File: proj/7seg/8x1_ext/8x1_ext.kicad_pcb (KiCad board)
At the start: 2 copper layers, 100 x 19 mm, 44 parts, among them J1 Conn_01x03_Pin, J2 grove, J3 UART, J4 UART, J9 USB_C, SW1 SW_Push, U1 74HC595, U10 D168K, U11 MCU_DISP, U12 MCU_CTL, U13 CH340E, U14 CH340K, U2 74HC595, U3 D168K, U4 D168K, U5 D168K, U6 D168K, U7 D168K, U8 D168K, U9 D168K

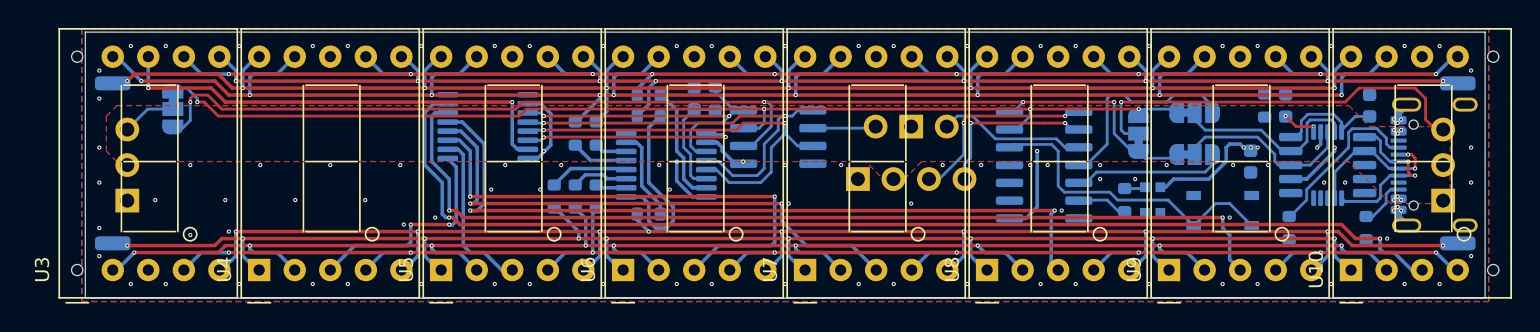
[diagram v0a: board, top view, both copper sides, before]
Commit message: -
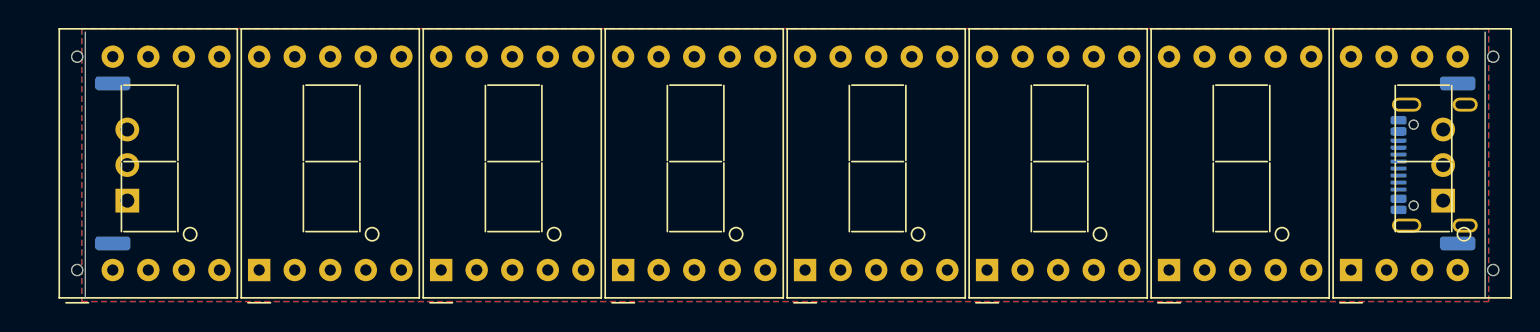
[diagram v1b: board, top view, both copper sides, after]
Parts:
- removed ?: , Library:PCB.MCBEERINGI.DEV
- removed C1: 0.1u, Capacitor_SMD:C_0603_1608Metric
- removed C2: 1u, Capacitor_SMD:C_0603_1608Metric
- removed C3: 0u1, Capacitor_SMD:C_0603_1608Metric
- removed D1: NeoPixel, LED_SMD:LED_WS2812B-2020_PLCC4_2.0x2.0mm
- removed D3: LED_TNOW, LED_SMD:LED_0603_1608Metric
- removed J1: Conn_01x03_Pin, Connector_PinHeader_2.54mm:PinHeader_1x03_P2.54mm_Vertical
- removed J2: grove, Connector_PinHeader_2.54mm:PinHeader_1x04_P2.54mm_Vertical
- removed JP1, JP2: T:R, Jumper:SolderJumper-3_P1.3mm_Bridged12_RoundedPad1.0x1.5mm
- removed JP5, JP6: DISP:CTL, Jumper:SolderJumper-3_P1.3mm_Bridged12_RoundedPad1.0x1.5mm
- removed R1, R2, R3, R4, R5, R6, R7, R8: 1k, Resistor_SMD:R_0603_1608Metric
- removed R10, R11: 5k1, Resistor_SMD:R_0603_1608Metric
- removed R12, R13, R9: 10k, Resistor_SMD:R_0603_1608Metric
- removed SW1: SW_Push, Library:alps-skrp
- removed U1, U2: 74HC595, Package_SO:TSSOP-16_4.4x5mm_P0.65mm
- removed U11: MCU_DISP, Package_SO:SOIC-8_3.9x4.9mm_P1.27mm
- removed U12: MCU_CTL, Package_SO:SOIC-14_3.9x8.7mm_P1.27mm
- removed U13: CH340E, Package_SO:MSOP-10_3x3mm_P0.5mm
- removed U14: CH340K, Package_SO:SSOP-10-1EP_3.9x4.9mm_P1mm_EP2.1x3.3mm
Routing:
- net F: track 127.2 -> 0.00 mm, vias 9 -> 0
- net D: track 119.9 -> 0.00 mm, vias 9 -> 0
- net C: track 117.7 -> 0.00 mm, vias 8 -> 0
- net A: track 116.3 -> 0.00 mm, vias 9 -> 0
- net H: track 111.6 -> 0.00 mm, vias 9 -> 0
- net G: track 109.4 -> 0.00 mm, vias 8 -> 0
- net E: track 109.2 -> 0.00 mm, vias 9 -> 0
- net B: track 105.6 -> 0.00 mm, vias 9 -> 0
- net RXD_DISP: track 83.2 -> 0.00 mm, vias 4 -> 0
- net C7: track 81.8 -> 0.00 mm, vias 2 -> 0
- net TXD_DISP: track 78.8 -> 0.00 mm, vias 4 -> 0
- net C6: track 68.2 -> 0.00 mm, vias 2 -> 0
- net C5: track 55.0 -> 0.00 mm, vias 2 -> 0
- net C4: track 38.7 -> 0.00 mm, vias 2 -> 0
- net C3: track 36.8 -> 0.00 mm, vias 2 -> 0
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- removed copper zone on F.Cu, net VCC
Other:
- board text removed: "7seg *8 dev board"
- board text removed: "AVR_CTL"
- board text removed: "AVR_DISP"
- board text removed: "CH340"
- board text removed: "CTR:DISP"
- board text removed: "C_V3"
- board text removed: "C_VCC"
- board text removed: "DR_TNOW"
- board text removed: "GND VCC SDA SCL"
- board text removed: "PA3"
- board text removed: "PA7"
- board text removed: "R:T"
- board text removed: "R_CC *2"
- board text removed: "T:R"
- board text removed: "UPDI GND UPDI"
